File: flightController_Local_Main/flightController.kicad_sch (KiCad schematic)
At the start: 27 parts, among them J1 U.FL-R-SMT10, J2 Conn_ARM_SWD, J3 USBC, U2 TESEO-LIV3F, U3 DPS368XTSA1, U4 STM32H723VETx, U6 TPS562201DDCR

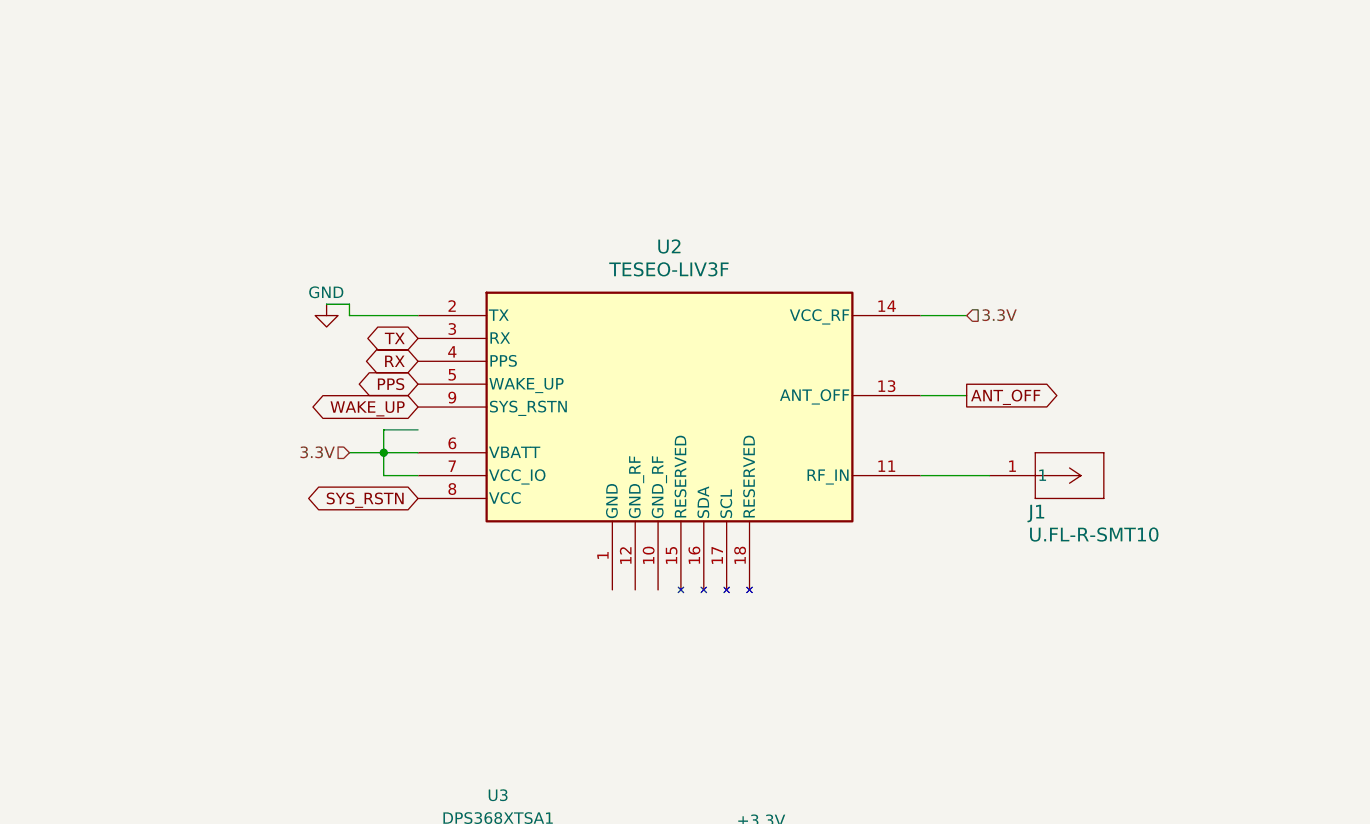
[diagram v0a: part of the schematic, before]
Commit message: Making changes to GPS
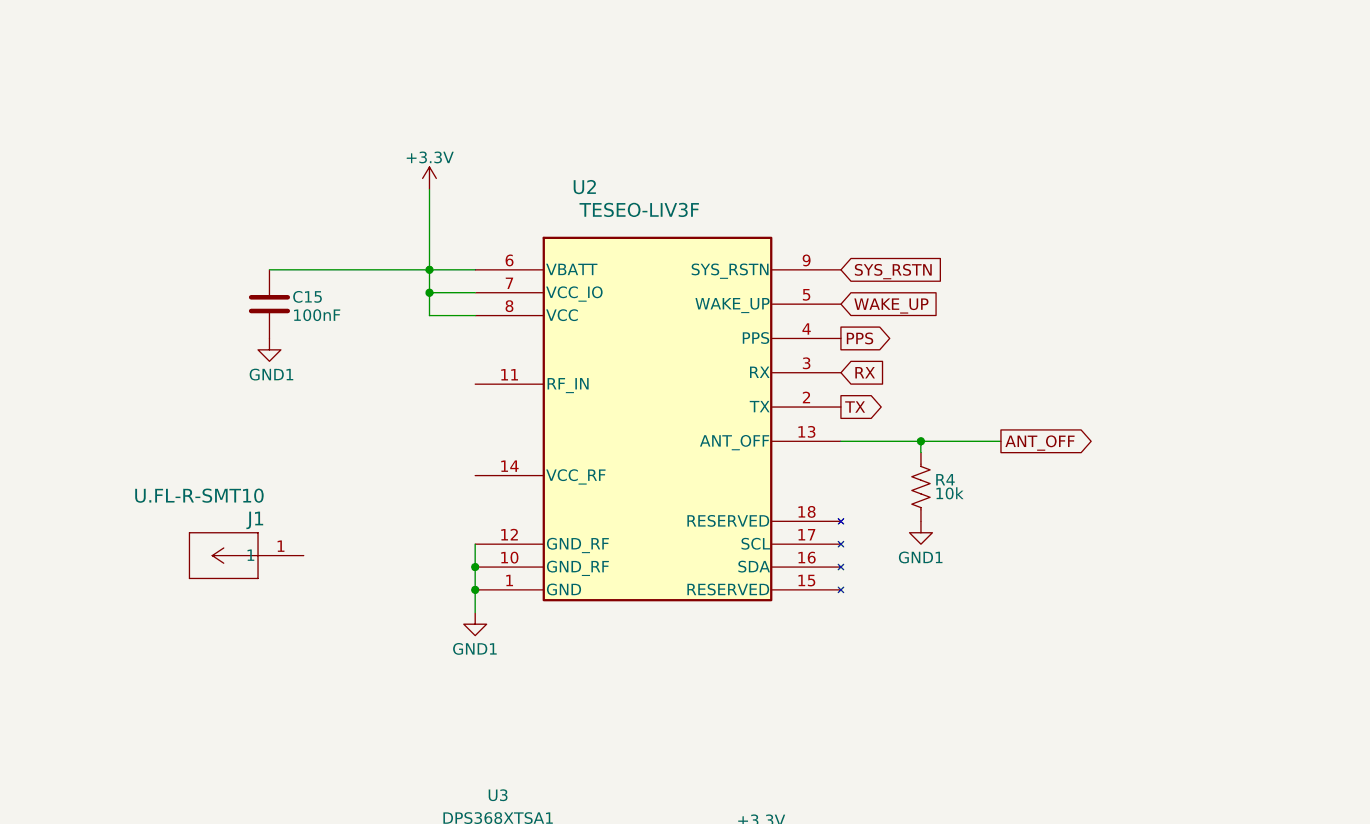
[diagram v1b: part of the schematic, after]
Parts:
- added C15: 100nF, symbol Device:C
- added R4: 10k, symbol Device:R_US
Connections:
- net +3.3V: now also U2.6 (VBATT), U2.7 (VCC_IO), U2.8 (VCC), C15.1
- net ANT_OFF: now also R4.1
- net GND: no longer U2.2 (TX)
- net GND1: now also U2.1 (GND), U2.10 (GND_RF), U2.12 (GND_RF), C15.2, R4.2
- net PPS: now also U2.4 (PPS); no longer U2.5 (WAKE_UP)
- net RX: now also U2.3 (RX); no longer U2.4 (PPS)
- net SYS_RSTN: now also U2.9 (SYS_RSTN); no longer U2.8 (VCC)
- net TX: now also U2.2 (TX); no longer U2.3 (RX)
- net WAKE_UP: now also U2.5 (WAKE_UP); no longer U2.9 (SYS_RSTN)
- net at J1.1: no longer U2.11 (RF_IN)
- removed net 3.3V: U2.14 (VCC_RF), U2.6 (VBATT), U2.7 (VCC_IO)
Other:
- moved on the sheet: J1, U2
